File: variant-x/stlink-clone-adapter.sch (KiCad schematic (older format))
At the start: 7 parts, among them J1 Conn_01x04, J2 Conn_01x04, J3 2X5_HDR, J4 Conn_01x04, J5 ARM_10PIN

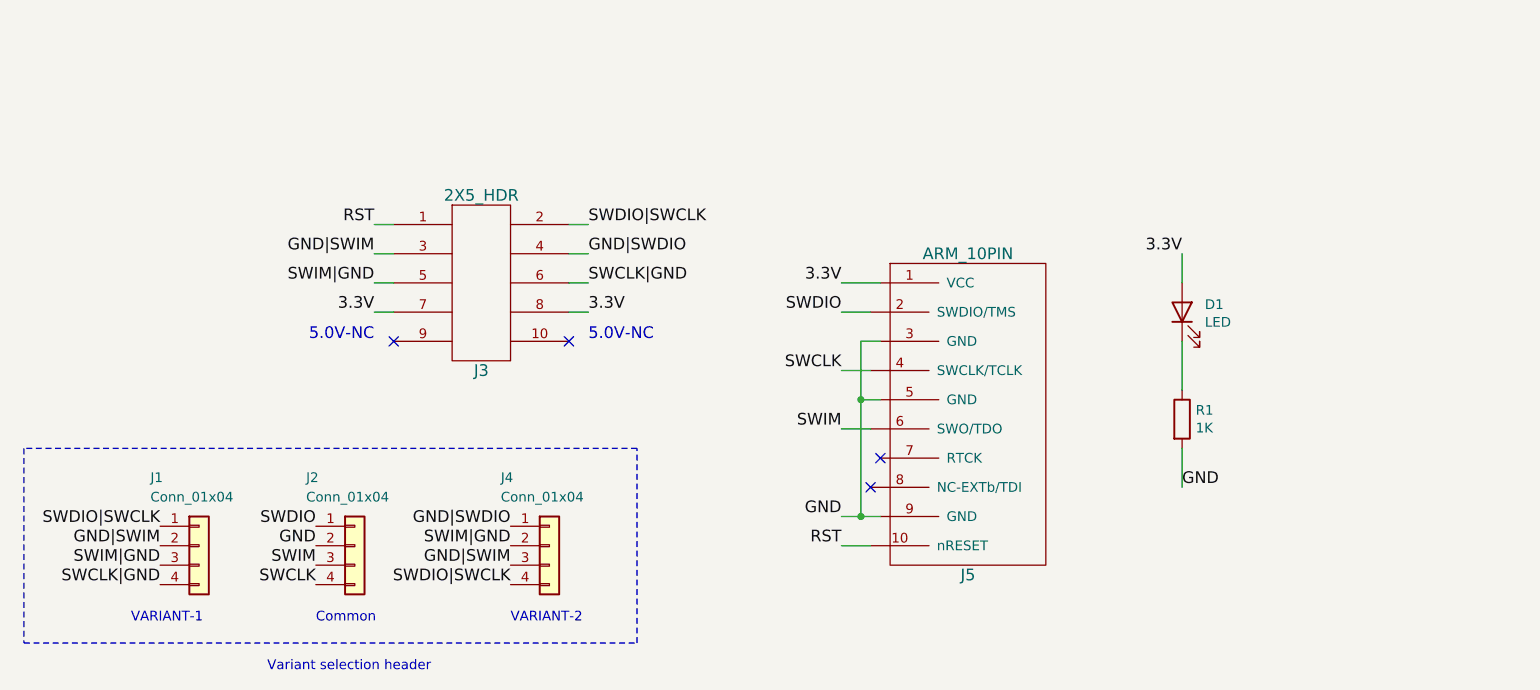
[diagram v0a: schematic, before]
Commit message: kibot
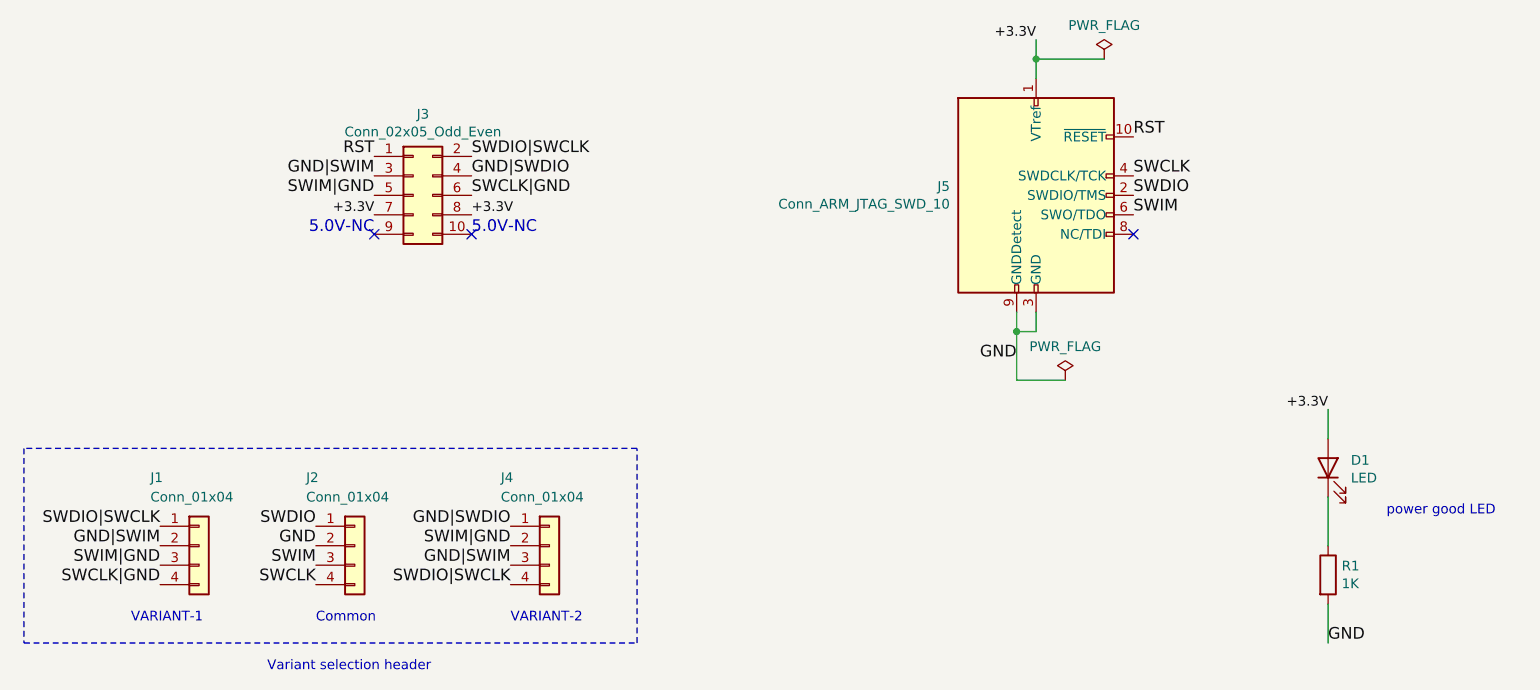
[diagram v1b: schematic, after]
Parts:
- removed J3: 2X5_HDR, Connector_PinSocket_2.54mm:PinSocket_2x05_P2.54mm_Horizontal, symbol stlink-clone-adapter-rescue:2X5_HDR-kicadlib-stlink-clone-adapter-rescue
- removed J5: ARM_10PIN, kicadlib:ARM_10_PIN, symbol stlink-clone-adapter-rescue:ARM_10PIN-kicadlib-stlink-clone-adapter-rescue
- added J3: Conn_02x05_Odd_Even, Connector_PinSocket_2.54mm:PinSocket_2x05_P2.54mm_Horizontal, symbol Connector_Generic:Conn_02x05_Odd_Even
- added J5: Conn_ARM_JTAG_SWD_10, kicadlib:ARM_10_PIN, symbol Connector:Conn_ARM_JTAG_SWD_10
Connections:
- net GND: now also J5.3 (GND), J5.5 (GND), J5.9 (GNDDetect)
- net GND|SWDIO: now also J3.4 (Pin_4)
- net GND|SWIM: now also J3.3 (Pin_3)
- net RST: now also J3.1 (Pin_1), J5.10 (~RESET~)
- net SWCLK: now also J5.4 (SWDCLK/TCK)
- net SWCLK|GND: now also J3.6 (Pin_6)
- net SWDIO: now also J5.2 (SWDIO/TMS)
- net SWDIO|SWCLK: now also J3.2 (Pin_2)
- net SWIM: now also J5.6 (SWO/TDO)
- net SWIM|GND: now also J3.5 (Pin_5)
- net 3.3V renamed +3.3V
- net +3.3V: now also J3.7 (Pin_7), J3.8 (Pin_8), J5.1 (VTref)
- no-connect marks 4 -> 3
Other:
- note added: "power good LED"
- moved on the sheet: D1, R1
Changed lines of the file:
@@
 Comment4 ""
 $EndDescr
-$Comp
-L stlink-clone-adapter-rescue:ARM_10PIN-kicadlib-stlink-clone-adapter-rescue J5
-U 1 1 5643BF5B
-P 7300 3300
-F 0 "J5" H 7300 2300 60  0000 C CNN
-F 1 "ARM_10PIN" H 7300 3950 60  0000 C CNN
-F 2 "kicadlib:ARM_10_PIN" H 7300 3300 60  0001 C CNN
-F 3 "" H 7300 3300 60  0000 C CNN
-	1    7300 3300
-	-1   0    0    -1
-$EndComp
-Text Label 4250 2500 2    60   ~ 0
+Text Label 4250 2150 2    60   ~ 0
 RST
-Text Label 5350 2650 0    60   ~ 0
+Text Label 4750 2250 0    60   ~ 0
 GND|SWDIO
-Text Label 5350 2800 0    60   ~ 0
+Text Label 4750 2350 0    60   ~ 0
 SWCLK|GND
-Text Label 4250 2800 2    60   ~ 0
+Text Label 4250 2350 2    60   ~ 0
 SWIM|GND
-Text Label 4250 2650 2    60   ~ 0
+Text Label 4250 2250 2    60   ~ 0
 GND|SWIM
-Text Label 5350 2500 0    60   ~ 0
+Text Label 4750 2150 0    60   ~ 0
 SWDIO|SWCLK
-Text Label 5350 2950 0    60   ~ 0
-3.3V
-Text Label 4250 2950 2    60   ~ 0
-3.3V
-Wire Wire Line
-	4250 2500 4350 2500
-Wire Wire Line
-	4250 2650 4350 2650
-Wire Wire Line
-	4250 2800 4350 2800
-Wire Wire Line
-	4250 2950 4350 2950
-Wire Wire Line
-	5350 2500 5250 2500
-Wire Wire Line
-	5250 2650 5350 2650
-Wire Wire Line
-	5350 2800 5250 2800
-Wire Wire Line
-	5250 2950 5350 2950
-Text Label 6650 2800 2    60   ~ 0
-3.3V
-Wire Wire Line
-	6650 2800 6850 2800
-NoConn ~ 5250 3100
-NoConn ~ 4350 3100
-Text Notes 5350 3100 0    60   ~ 0
+NoConn ~ 4750 2550
+NoConn ~ 4250 2550
+Text Notes 4750 2550 0    60   ~ 0
 5.0V-NC
-Text Notes 4250 3100 2    60   ~ 0
+Text Notes 4250 2550 2    60   ~ 0
 5.0V-NC
-Text Label 6650 2950 2    60   ~ 0
+Text Label 8150 2350 0    60   ~ 0
 SWDIO
-Text Label 6650 4000 2    60   ~ 0
+Text Label 7550 3200 2    60   ~ 0
 GND
-Wire Wire Line
-	6650 4000 6750 4000
-Wire Wire Line
-	6850 3400 6750 3400
-Wire Wire Line
-	6750 3100 6750 3400
-Connection ~ 6750 4000
-Wire Wire Line
-	6850 3100 6750 3100
-Connection ~ 6750 3400
-NoConn ~ 6800 3850
-NoConn ~ 6850 3700
-Text Label 6650 4150 2    60   ~ 0
+Text Label 8150 2050 0    60   ~ 0
 RST
-Text Label 6650 3550 2    60   ~ 0
+Text Label 8150 2450 0    60   ~ 0
 SWIM
-Text Label 6650 3250 2    60   ~ 0
+Text Label 8150 2250 0    60   ~ 0
 SWCLK
-Wire Wire Line
-	6650 2950 6800 2950
-Wire Wire Line
-	6800 3250 6650 3250
-Wire Wire Line
-	6650 3550 6800 3550
-Wire Wire Line
-	6800 4150 6650 4150
-$Comp
-L stlink-clone-adapter-rescue:2X5_HDR-kicadlib-stlink-clone-adapter-rescue J3
-U 1 1 5643C704
-P 4800 2750
-F 0 "J3" H 4800 2250 60  0000 C CNN
-F 1 "2X5_HDR" H 4800 3150 60  0000 C CNN
-F 2 "Connector_PinSocket_2.54mm:PinSocket_2x05_P2.54mm_Horizontal" H 4700 2500 60  0001 C CNN
-F 3 "" H 4700 2500 60  0000 C CNN
-	1    4800 2750
-	1    0    0    -1
-$EndComp
-Wire Wire Line
-	6750 4000 6850 4000
-Wire Wire Line
-	6750 3400 6750 4000
 Text Label 3950 4050 2    60   ~ 0
 SWDIO
@@
 L Device:LED D1
 U 1 1 5FDE2375
-P 8400 2950
-F 0 "D1" V 8439 2833 50  0000 R CNN
-F 1 "LED" V 8348 2833 50  0000 R CNN
-F 2 "LED_SMD:LED_0603_1608Metric" H 8400 2950 50  0001 C CNN
-F 3 "~" H 8400 2950 50  0001 C CNN
-	1    8400 2950
+P 9150 3750
+F 0 "D1" V 9189 3633 50  0000 R CNN
+F 1 "LED" V 9098 3633 50  0000 R CNN
+F 2 "LED_SMD:LED_0603_1608Metric" H 9150 3750 50  0001 C CNN
+F 3 "~" H 9150 3750 50  0001 C CNN
+	1    9150 3750
 	0    -1   -1   0
 $EndComp
@@
 L Device:R R1
 U 1 1 5FDE299C
-P 8400 3500
-F 0 "R1" H 8470 3546 50  0000 L CNN
-F 1 "1K" H 8470 3455 50  0000 L CNN
-F 2 "Resistor_SMD:R_0603_1608Metric" V 8330 3500 50  0001 C CNN
-F 3 "~" H 8400 3500 50  0001 C CNN
-	1    8400 3500
-	1    0    0    -1
-$EndComp
-Text Label 8400 3850 0    60   ~ 0
+P 9150 4300
+F 0 "R1" H 9220 4346 50  0000 L CNN
+F 1 "1K" H 9220 4255 50  0000 L CNN
+F 2 "Resistor_SMD:R_0603_1608Metric" V 9080 4300 50  0001 C CNN
+F 3 "~" H 9150 4300 50  0001 C CNN
+	1    9150 4300
+	1    0    0    -1
+$EndComp
+Text Label 9150 4650 0    60   ~ 0
 GND
 Wire Wire Line
-	8400 3850 8400 3650
-Wire Wire Line
-	8400 3350 8400 3100
-Text Label 8400 2650 2    60   ~ 0
-3.3V
-Wire Wire Line
-	8400 2650 8400 2800
+	9150 4650 9150 4450
+Wire Wire Line
+	9150 4150 9150 3900
+Wire Wire Line
+	9150 3450 9150 3600
+$Comp
+L Connector_Generic:Conn_02x05_Odd_Even J3
+U 1 1 5FE390A4
+P 4450 2350
+F 0 "J3" H 4500 2767 50  0000 C CNN
+F 1 "Conn_02x05_Odd_Even" H 4500 2676 50  0000 C CNN
+F 2 "Connector_PinSocket_2.54mm:PinSocket_2x05_P2.54mm_Horizontal" H 4450 2350 50  0001 C CNN
+F 3 "~" H 4450 2350 50  0001 C CNN
+	1    4450 2350
+	1    0    0    -1
+$EndComp
+$Comp
+L Connector:Conn_ARM_JTAG_SWD_10 J5
+U 1 1 5FE5000B
+P 7650 2350
+F 0 "J5" H 7207 2396 50  0000 R CNN
+F 1 "Conn_ARM_JTAG_SWD_10" H 7207 2305 50  0000 R CNN
+F 2 "kicadlib:ARM_10_PIN" H 7650 2350 50  0001 C CNN
+F 3 "http://infocenter.arm.com/help/topic/com.arm.doc.ddi0314h/DDI0314H_coresight_components_trm.pdf" V 7300 1100 50  0001 C CNN
+	1    7650 2350
+	1    0    0    -1
+$EndComp
+Wire Wire Line
+	7550 2950 7550 3050
+Wire Wire Line
+	7650 2950 7650 3050
+Wire Wire Line
+	7650 3050 7550 3050
+Connection ~ 7550 3050
+Text Notes 9450 4000 0    50   ~ 0
+power good LED
+NoConn ~ 8150 2550
+Wire Wire Line
+	7650 1550 7650 1650
+$Comp
+L power:PWR_FLAG #FLG0101
+U 1 1 5FE6AB4B
+P 8000 1650
+F 0 "#FLG0101" H 8000 1725 50  0001 C CNN
+F 1 "PWR_FLAG" H 8000 1823 50  0000 C CNN
+F 2 "" H 8000 1650 50  0001 C CNN
+F 3 "~" H 8000 1650 50  0001 C CNN
+	1    8000 1650
+	1    0    0    -1
+$EndComp
+Wire Wire Line
+	8000 1650 7650 1650
+Connection ~ 7650 1650
+Wire Wire Line
+	7650 1650 7650 1750
+Wire Wire Line
+	7550 3300 7800 3300
+Wire Wire Line
+	7550 3050 7550 3300
+$Comp
+L power:PWR_FLAG #FLG0102
+U 1 1 5FE6C1C4
+P 7800 3300
+F 0 "#FLG0102" H 7800 3375 50  0001 C CNN
+F 1 "PWR_FLAG" H 7800 3473 50  0000 C CNN
+F 2 "" H 7800 3300 50  0001 C CNN
+F 3 "~" H 7800 3300 50  0001 C CNN
+	1    7800 3300
+	1    0    0    -1
+$EndComp
+Text Label 9150 3450 2    50   ~ 0
++3.3V
+Text Label 7650 1550 2    50   ~ 0
++3.3V
+Text Label 4250 2450 2    50   ~ 0
++3.3V
+Text Label 4750 2450 0    50   ~ 0
++3.3V
 $EndSCHEMATC
